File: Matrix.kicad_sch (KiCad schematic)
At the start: 140 parts

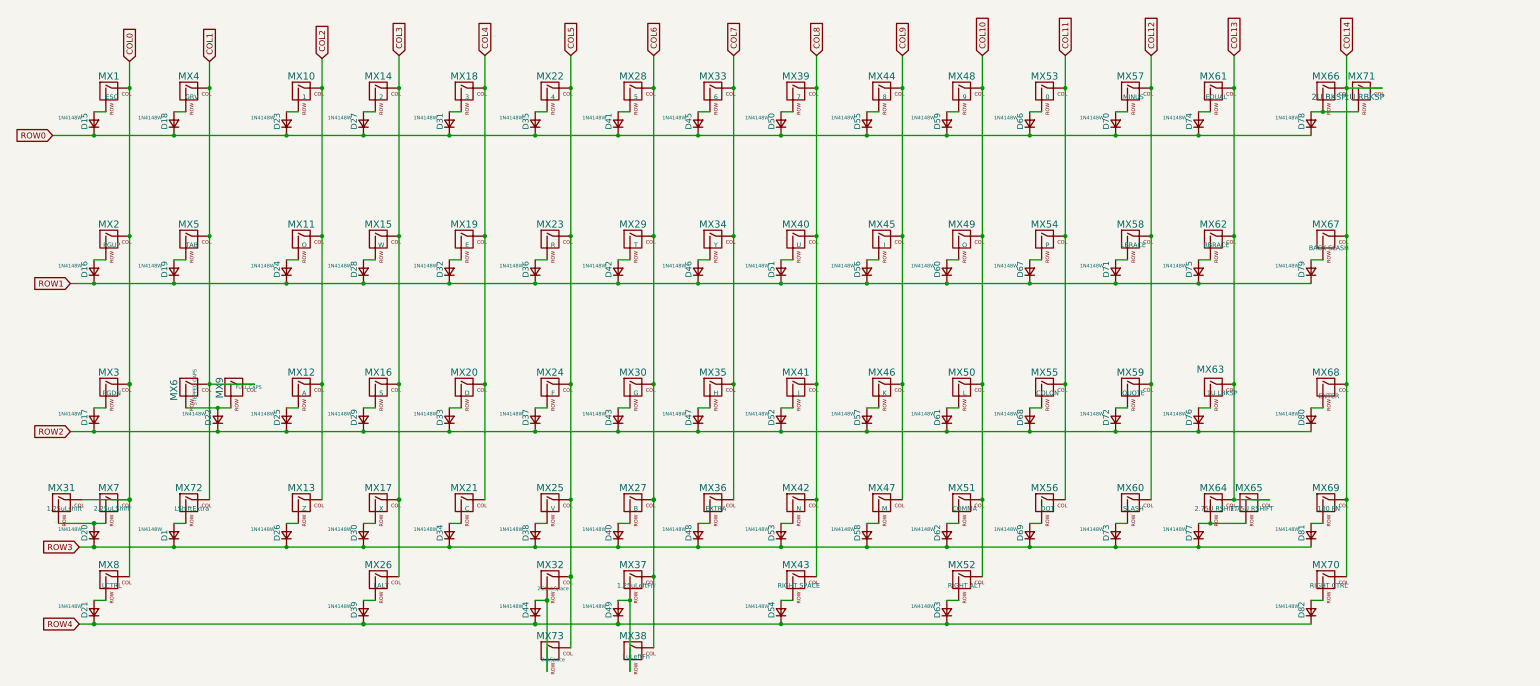
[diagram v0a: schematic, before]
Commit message: Updated things
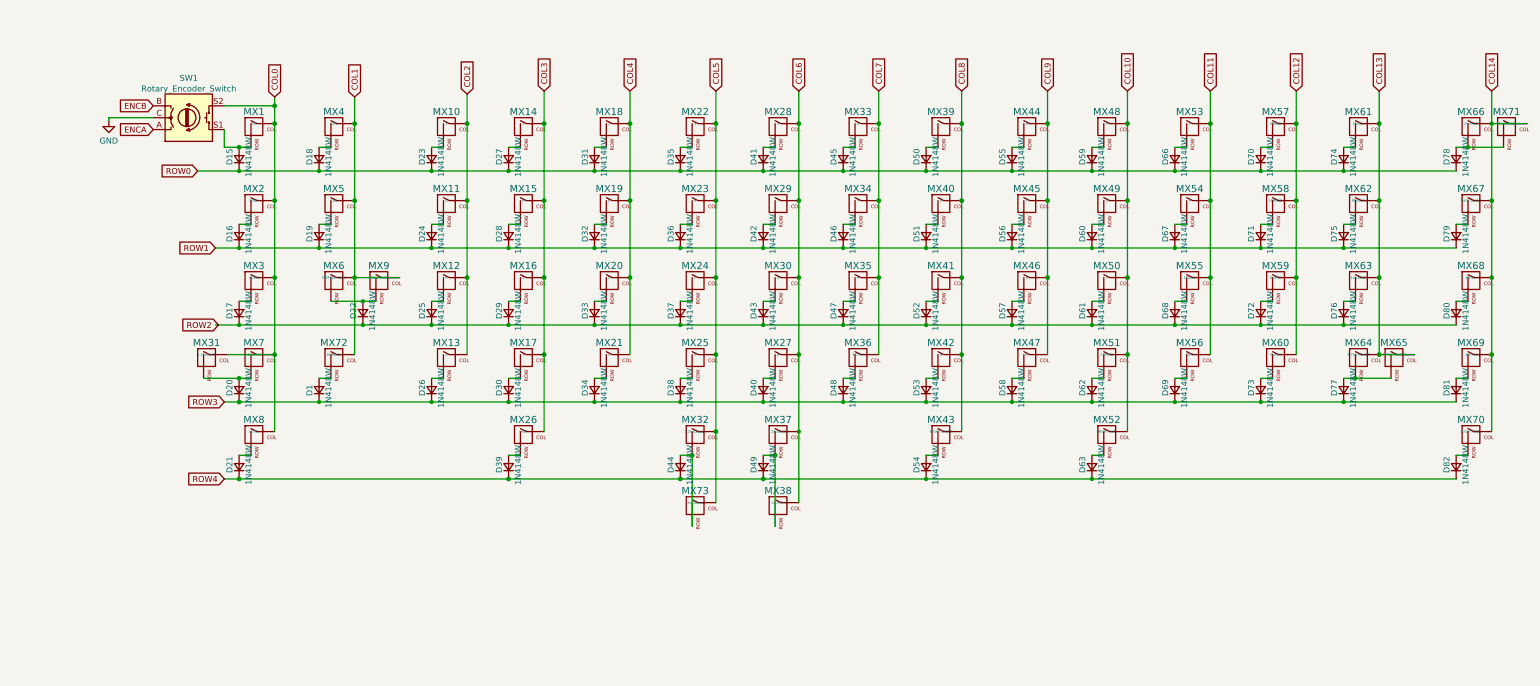
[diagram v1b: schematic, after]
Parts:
- added SW1: Rotary_Encoder_Switch, Keeb-IO:RotaryEncoder_Alps_EC11E-Switch_Vertical_H20mm, symbol Device:Rotary_Encoder_Switch
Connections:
- net COL0: now also SW1.S2
- net at D15.2 (A), MX1.2 (ROW): now also SW1.S1
- new net ENCA: SW1.A
- new net ENCB: SW1.B
- new net GND: SW1.C
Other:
- moved on the sheet: D1, D15, D16, D17, D18, D19, D20, D21, D22, D23, D24, D25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
